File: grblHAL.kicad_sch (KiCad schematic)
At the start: 49 parts, among them J1 Conn_01x03, J2 Conn_02x08_Odd_Even, J3 Conn_01x06, J4 Conn_01x06, J5 Conn_01x04, U1 YAAJ_BluePill_Part_Like_SWD_B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, U10 PC817, U11 PC817, U12 PC817, U13 PC817, U14 LM1117-3.3, U2 TMC2208_SILENTSTEPSTICK, U3 buck2596, U4 PC817, U5 PC817, U6 PC817, U7 PC817, U8 PC817, U9 PC817

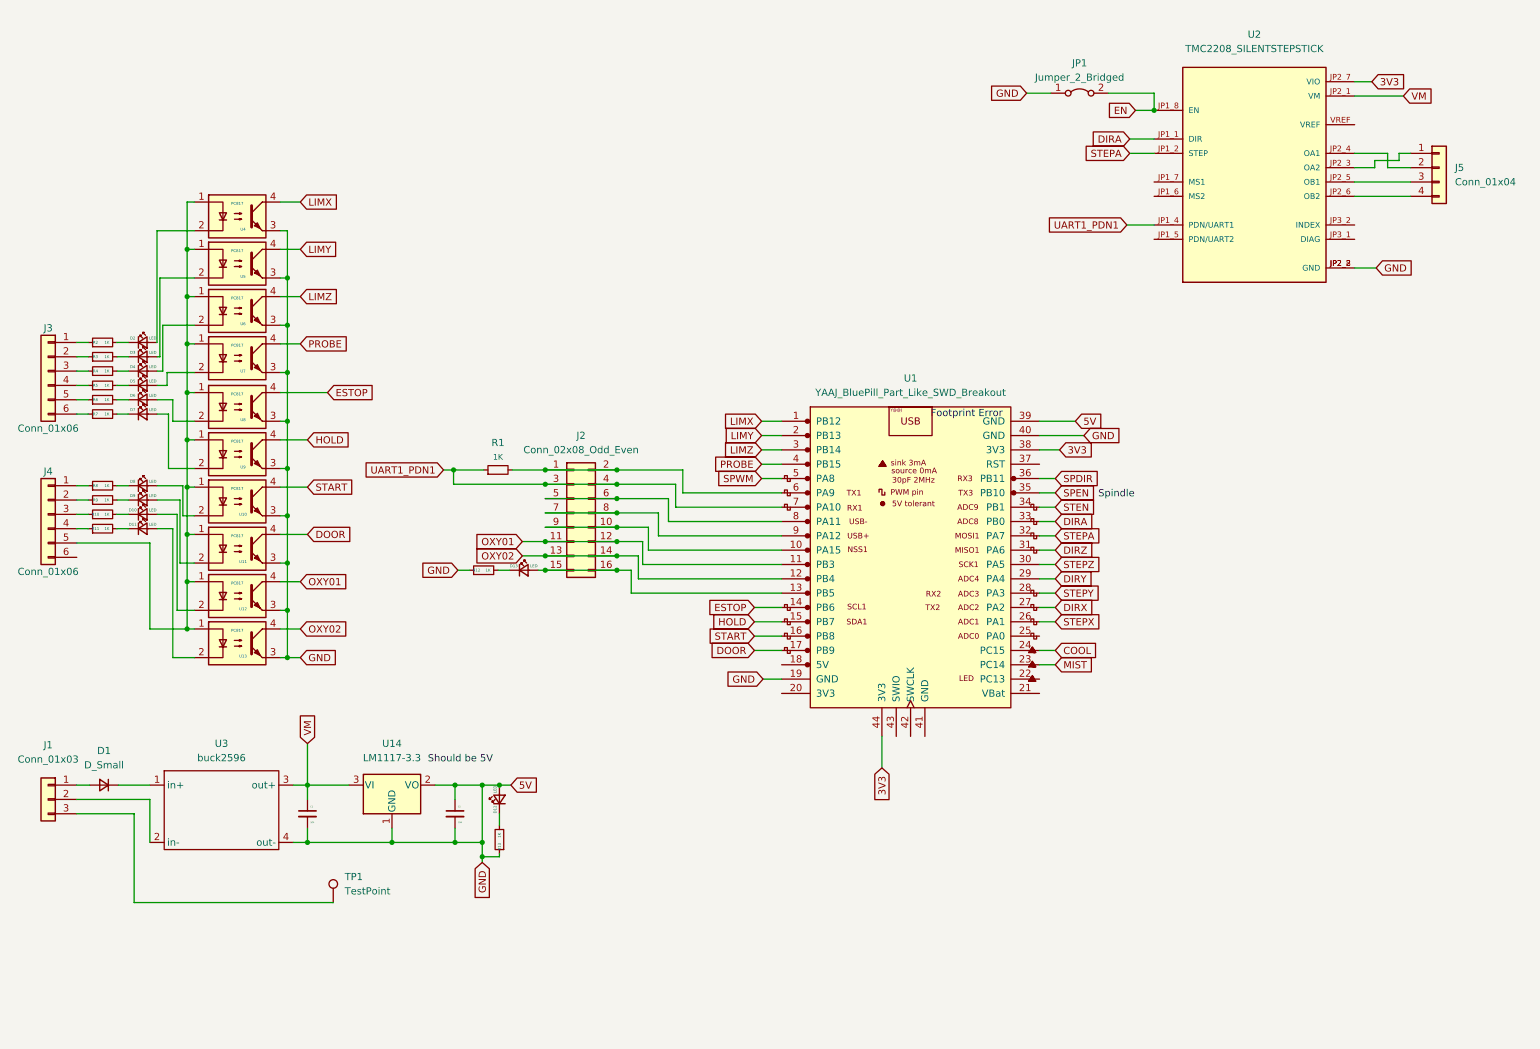
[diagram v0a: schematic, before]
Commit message: Schematic Layout Nets Opto 4 TMC Stage 2
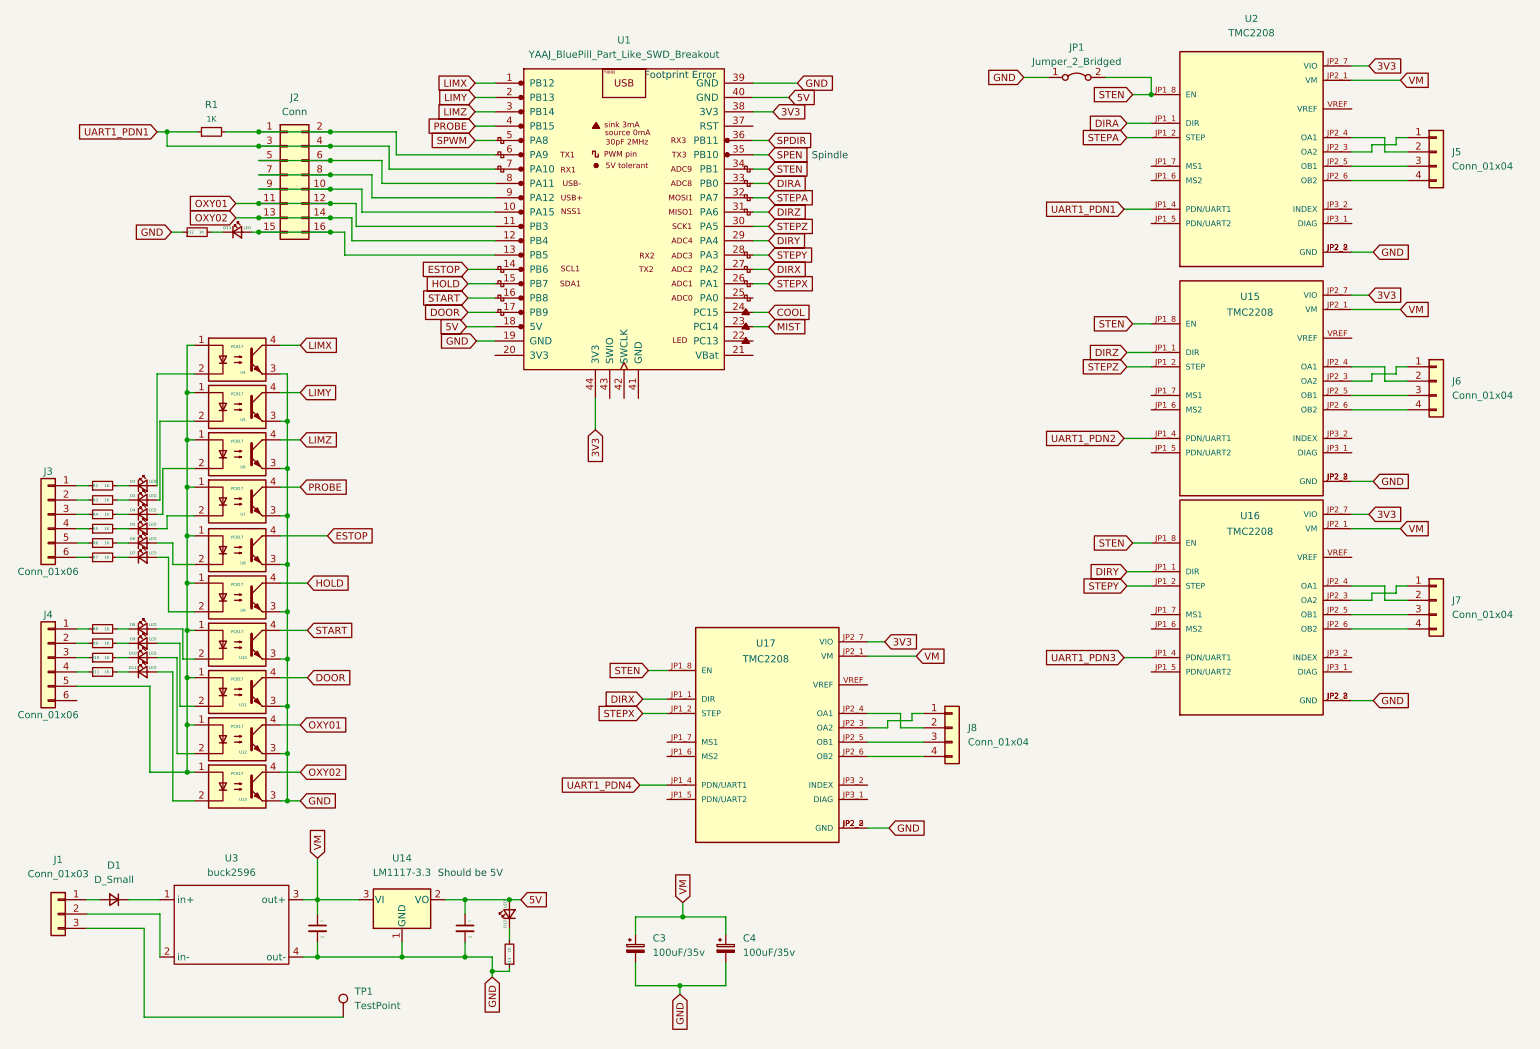
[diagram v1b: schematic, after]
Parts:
- added C3, C4: 100uF/35v, Capacitor_THT:CP_Radial_D8.0mm_P3.50mm, symbol Device:C_Polarized_Small
- added J6, J7, J8: Conn_01x04, Connector_PinHeader_2.54mm:PinHeader_1x04_P2.54mm_Vertical, symbol Connector_Generic:Conn_01x04
- added U15, U16, U17: TMC2208, TMC2208_SILENTSTEPSTICK:MODULE_TMC2208_SILENTSTEPSTICK, symbol TMC2208_SILENTSTEPSTICK:TMC2208_SILENTSTEPSTICK
- J2: value Conn_02x08_Odd_Even -> Conn
- J3, J4: footprint Connector_Phoenix_MC_HighVoltage:PhoenixContact_MC_1,5_6-G-5.08_1x06_P5.08mm_Horizontal -> Connector_Phoenix_MSTB:PhoenixContact_MSTBA_2,5_6-G-5,08_1x06_P5.08mm_Horizontal
- U2: value TMC2208_SILENTSTEPSTICK -> TMC2208
- U3: footprint Buck2596:buck2596 -> DC_DC_LM2596_small:DC_DC_LM2596_small
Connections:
- net EN is gone; now on net STEN: JP1.2 (B), U2.JP1_8 (EN)
- net 3V3: now also U15.JP2_7 (VIO), U16.JP2_7 (VIO), U17.JP2_7 (VIO)
- net 5V: now also U1.18 (5V); no longer C1.2, C2.2, JP1.1 (A), R12.1, R13.1, U1.19 (GND), U1.39 (GND), U10.3, U11.3, U12.3, U13.3, U14.1 (GND), U2.JP2_2 (GND), U2.JP2_8 (GND), U3.4 (out-), U4.3, U5.3, U6.3, U7.3, U8.3, U9.3
- net DIRX: now also U17.JP1_1 (DIR)
- net DIRY: now also U16.JP1_1 (DIR)
- net DIRZ: now also U15.JP1_1 (DIR)
- net STEN: now also U15.JP1_8 (EN), U16.JP1_8 (EN), U17.JP1_8 (EN)
- net STEPX: now also U17.JP1_2 (STEP)
- net STEPY: now also U16.JP1_2 (STEP)
- net STEPZ: now also U15.JP1_2 (STEP)
- net VM: now also C3.1, C4.1, U15.JP2_1 (VM), U16.JP2_1 (VM), U17.JP2_1 (VM)
- new net: J6.1 (Pin_1), U15.JP2_3 (OA2)
- new net: J6.2 (Pin_2), U15.JP2_4 (OA1)
- new net: J6.3 (Pin_3), U15.JP2_5 (OB1)
- new net: J6.4 (Pin_4), U15.JP2_6 (OB2)
- new net: J7.1 (Pin_1), U16.JP2_3 (OA2)
- new net: J7.2 (Pin_2), U16.JP2_4 (OA1)
- new net: J7.3 (Pin_3), U16.JP2_5 (OB1)
- new net: J7.4 (Pin_4), U16.JP2_6 (OB2)
- new net: J8.1 (Pin_1), U17.JP2_3 (OA2)
- new net: J8.2 (Pin_2), U17.JP2_4 (OA1)
- new net: J8.3 (Pin_3), U17.JP2_5 (OB1)
- new net: J8.4 (Pin_4), U17.JP2_6 (OB2)
- new net GND: C1.2, C2.2, C3.2, C4.2, JP1.1 (A), R12.1, R13.1, U1.19 (GND), U1.39 (GND), U10.3, U11.3, U12.3, U13.3, U14.1 (GND), U15.JP2_2 (GND), U15.JP2_8 (GND), U16.JP2_2 (GND), U16.JP2_8 (GND), U17.JP2_2 (GND), U17.JP2_8 (GND), U2.JP2_2 (GND), U2.JP2_8 (GND), U3.4 (out-), U4.3, U5.3, U6.3, U7.3, U8.3, U9.3
- new net UART1_PDN2: U15.JP1_4 (PDN/UART1)
- new net UART1_PDN3: U16.JP1_4 (PDN/UART1)
- new net UART1_PDN4: U17.JP1_4 (PDN/UART1)
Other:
- moved on the sheet: C1, C2, D1, D10, D11, D12, D13, D2, D3, D4, D5, D6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
